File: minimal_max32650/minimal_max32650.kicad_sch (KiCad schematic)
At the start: 57 parts, among them J1 FTSH-105-01-L-DV-K, Q1 50 V, Q2 50 V, U1 ADT75BRMZ, U2 MX25U6432FZNI02, U3 MAX32650GCE+, U4 MAXQ1065GTC+, U5 ADP225ACPZ-R7

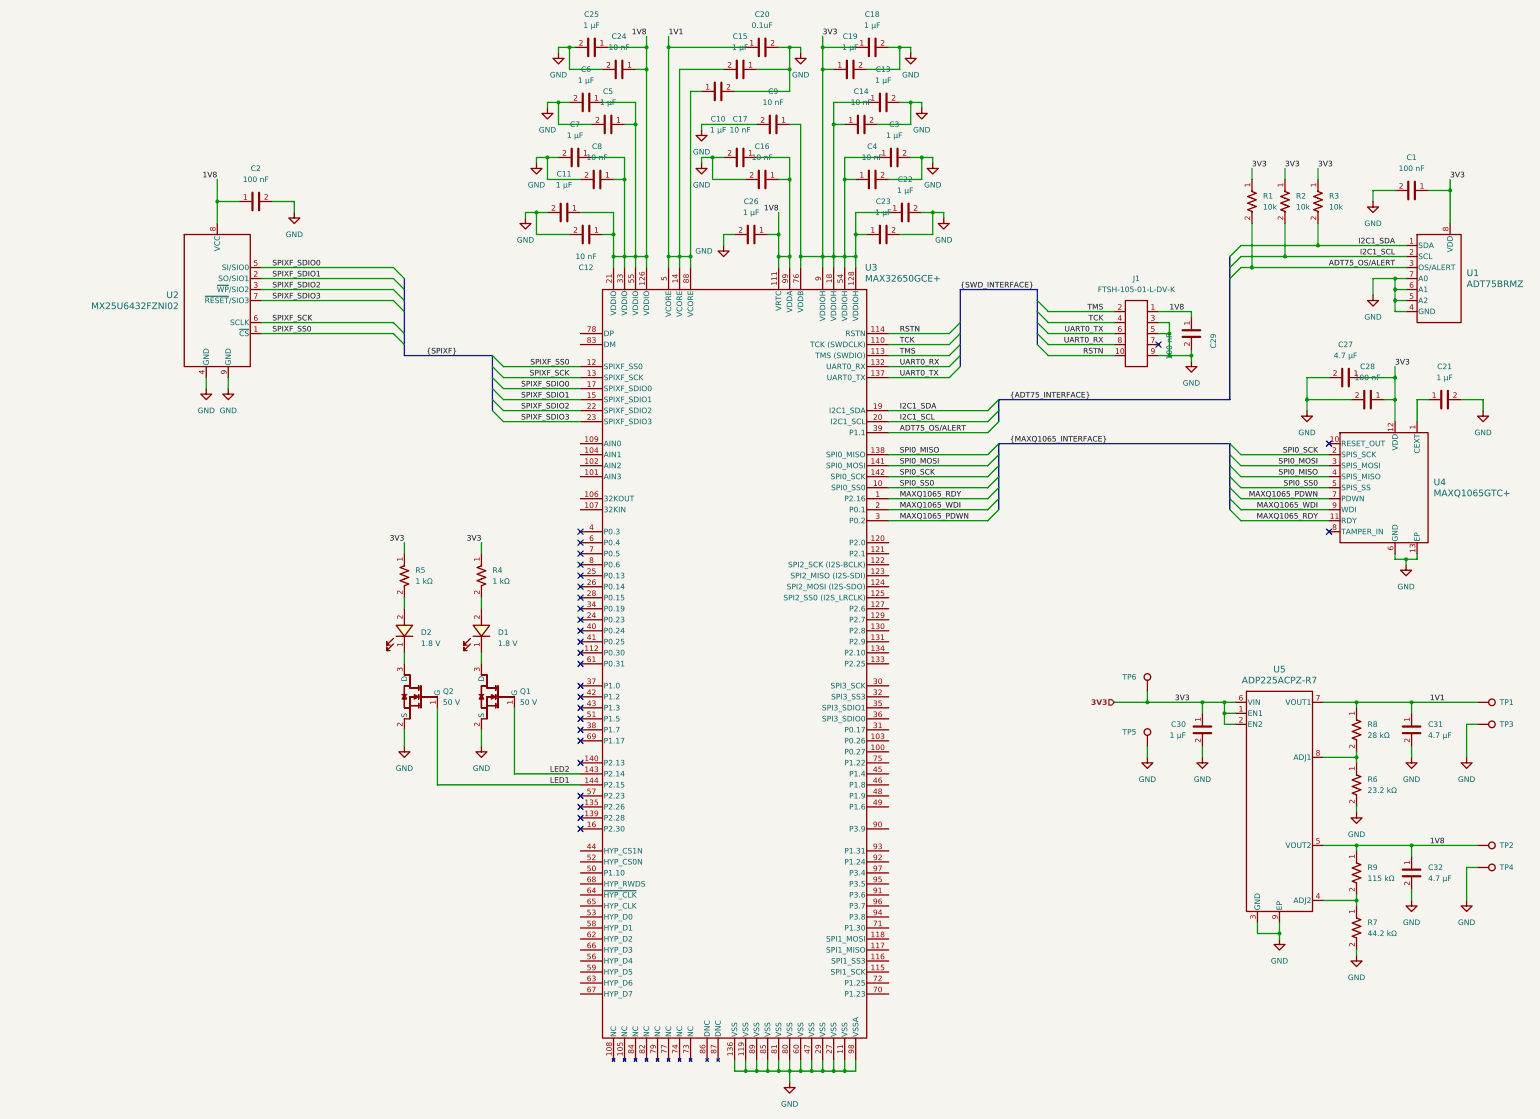
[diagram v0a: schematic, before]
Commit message: development backup
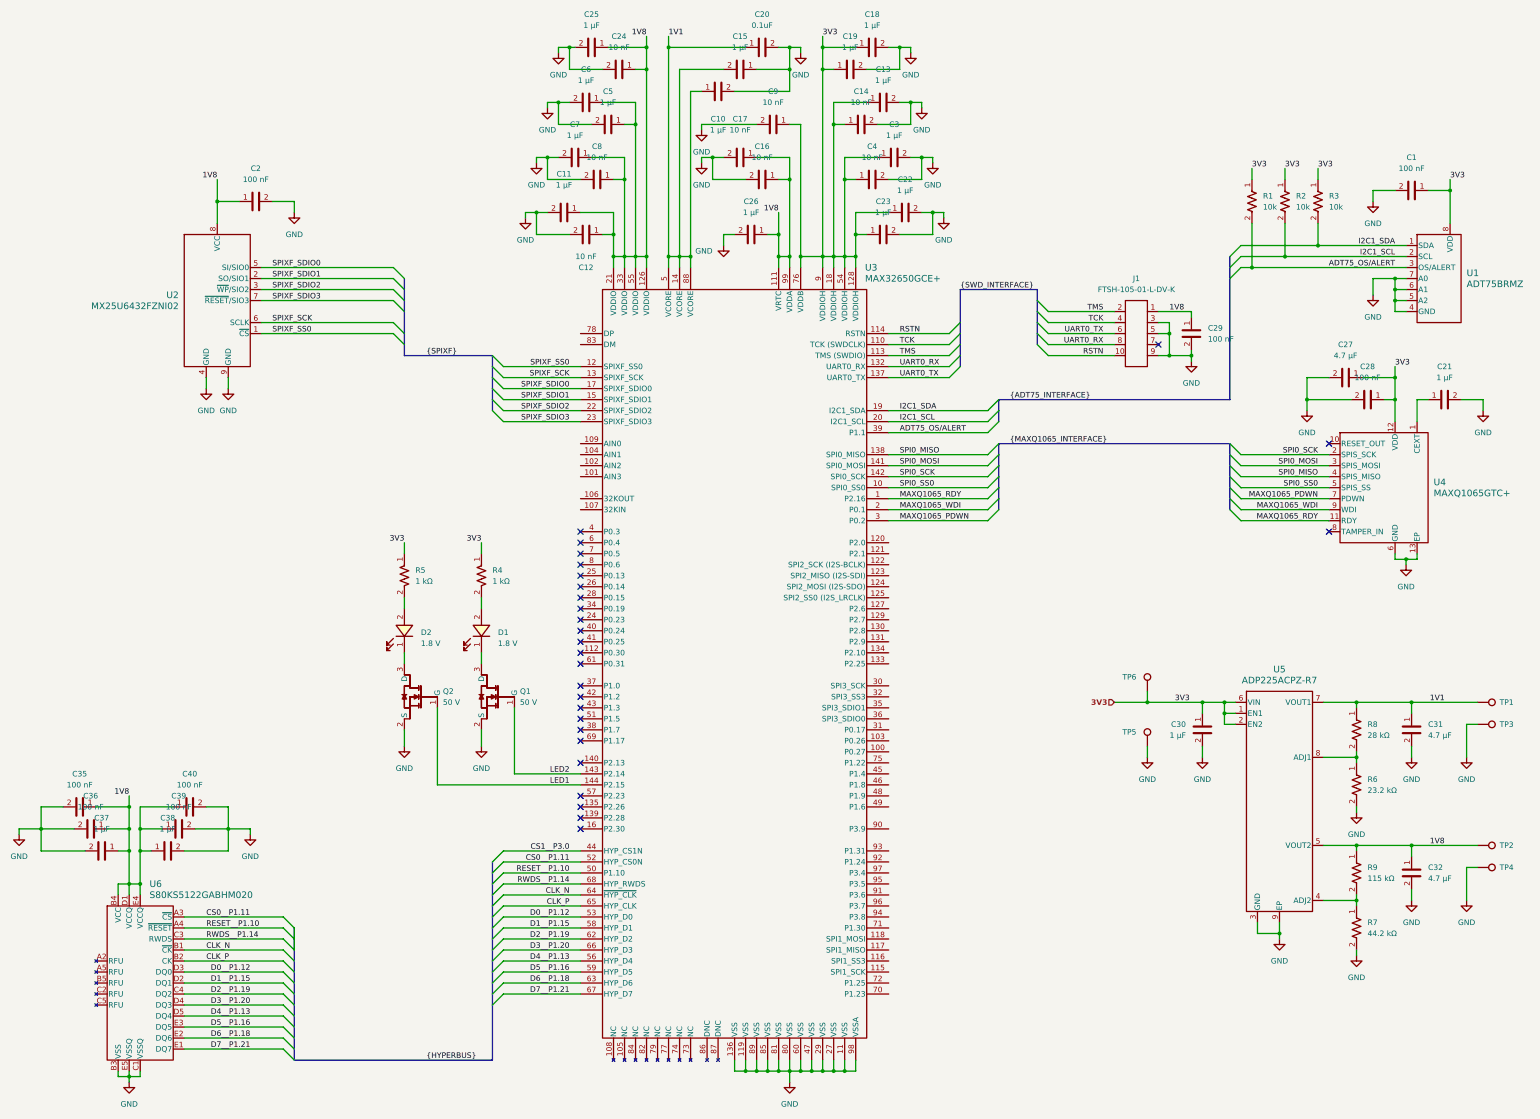
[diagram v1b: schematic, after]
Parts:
- added C35, C36, C39, C40: 100 nF, capacitor_footprints:C_0402_1005Metric, symbol UNITED_CAPACITORS_DATA_BASE:C_GCM155R71H104KE02D
- added C37, C38: 1 µF, capacitor_footprints:C_0402_1005Metric, symbol UNITED_CAPACITORS_DATA_BASE:C_C1005X6S1C105K050BC
- added U6: S80KS5122GABHM020, infineon_footprints:PG-BGA-24-801, symbol UNITED_IC_INFINEON:U_S80KS5122GABHM020
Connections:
- net 1V8: now also C35.1, C36.1, C37.1, C38.1, C39.1, C40.1, U6.B4 (VCC), U6.D1 (VCCQ), U6.E4 (VCCQ)
- net GND: now also C35.2, C36.2, C37.2, C38.2, C39.2, C40.2, U6.B3 (VSS), U6.C1 (VSSQ), U6.E5 (VSSQ)
- net CS1__P3.0: now reaches U3.44 (P3.0)
- net RESET__P1.10: now reaches U3.50 (P1.10)
- net RESET__P1.10: now also U6.A4 (~{RESET})
- net CS0__P1.11: now reaches U3.52 (P1.11)
- net CS0__P1.11: now also U6.A3 (~{CS})
- net D0__P1.12: now reaches U3.53 (P1.12)
- net D0__P1.12: now also U6.D3 (DQ0)
- net D4__P1.13: now reaches U3.56 (P1.13)
- net D4__P1.13: now also U6.D5 (DQ4)
- net D1__P1.15: now reaches U3.58 (P1.15)
- net D1__P1.15: now also U6.D2 (DQ1)
- net D5__P1.16: now reaches U3.59 (P1.16)
- net D5__P1.16: now also U6.E3 (DQ5)
- net D2__P1.19: now reaches U3.62 (P1.19)
- net D2__P1.19: now also U6.C4 (DQ2)
- net D6__P1.18: now reaches U3.63 (P1.18)
- net D6__P1.18: now also U6.E2 (DQ6)
- net CLK_N: now reaches U3.64 (~{HYP_CLK})
- net CLK_N: now also U6.B1 (~{CK})
- net CLK_P: now reaches U3.65 (HYP_CLK)
- net CLK_P: now also U6.B2 (CK)
- net D3__P1.20: now reaches U3.66 (P1.20)
- net D3__P1.20: now also U6.D4 (DQ3)
- net D7__P1.21: now reaches U3.67 (P1.21)
- net D7__P1.21: now also U6.E1 (DQ7)
- net RWDS__P1.14: now reaches U3.68 (P1.14)
- net RWDS__P1.14: now also U6.C3 (RWDS)
